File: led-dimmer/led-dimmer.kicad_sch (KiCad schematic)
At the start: 14 parts, among them J1 Screw_Terminal_01x02, J2 Screw_Terminal_01x02, Q1 IRLML6344, U1 LM555xM

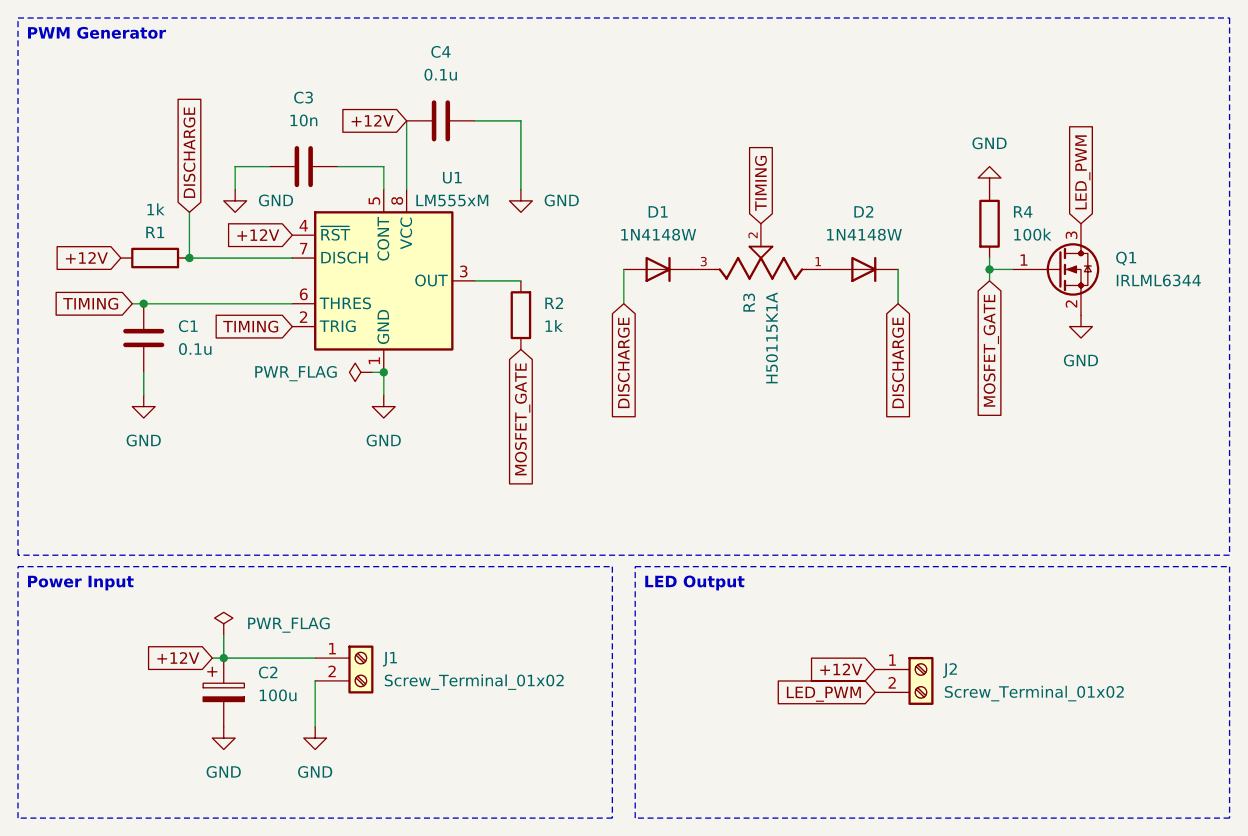
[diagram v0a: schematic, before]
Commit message: Update LED Dimmer PCB
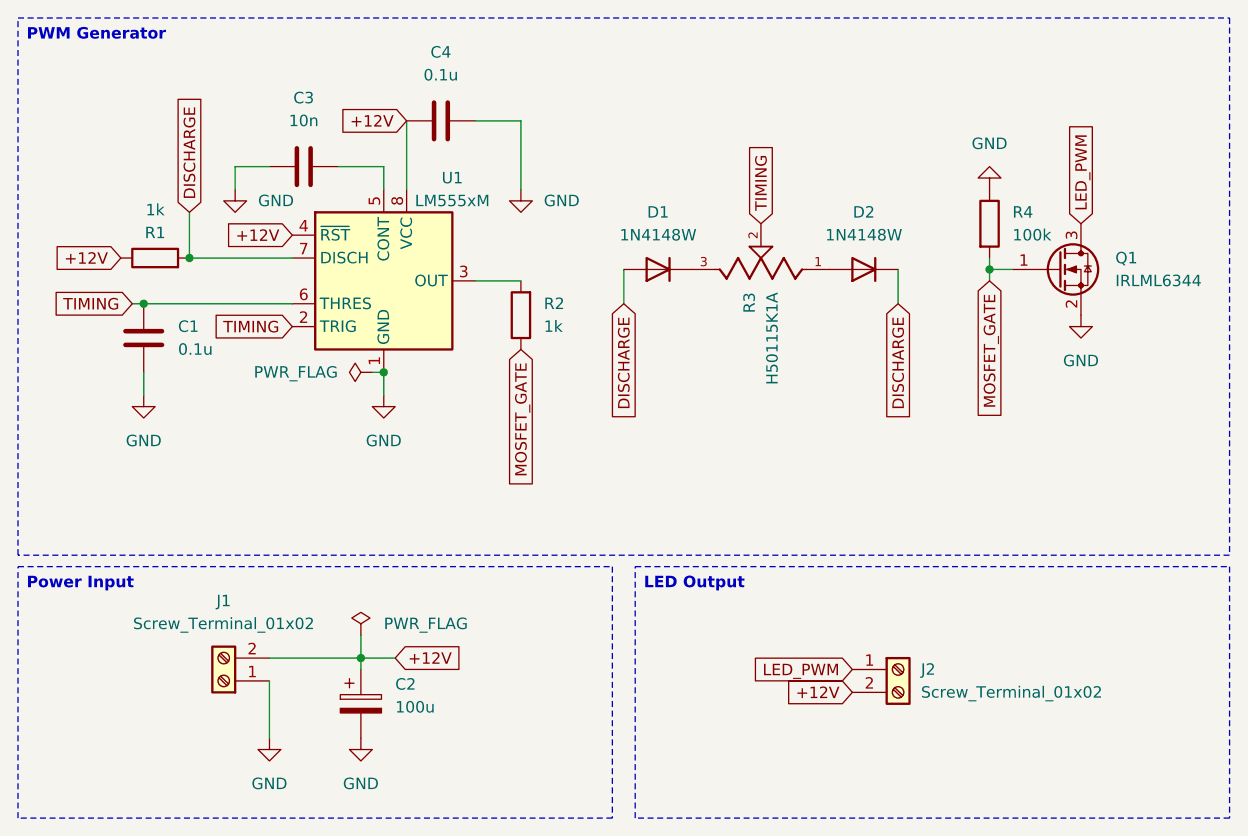
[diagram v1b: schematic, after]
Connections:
- net +12V: now also J1.2 (Pin_2), J2.2 (Pin_2); no longer J1.1 (Pin_1), J2.1 (Pin_1)
- net GND: now also J1.1 (Pin_1); no longer J1.2 (Pin_2)
- net LED_PWM: now also J2.1 (Pin_1); no longer J2.2 (Pin_2)
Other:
- moved on the sheet: C2, J1, J2
